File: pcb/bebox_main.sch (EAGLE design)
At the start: 29 parts, among them J1 SJ-435107RS, J2 SJ-435107RS, J4 SJ-435107RS, J6 PJ-102AH, P1 OSTTE020104, P2 OSTTE020104, P3 OSTTE020104, P4 OSTTE020104, P5 OSTTE020104, T1 TIP122, T2 TIP122, T3 TIP122, T4 TIP122, T5 TIP122

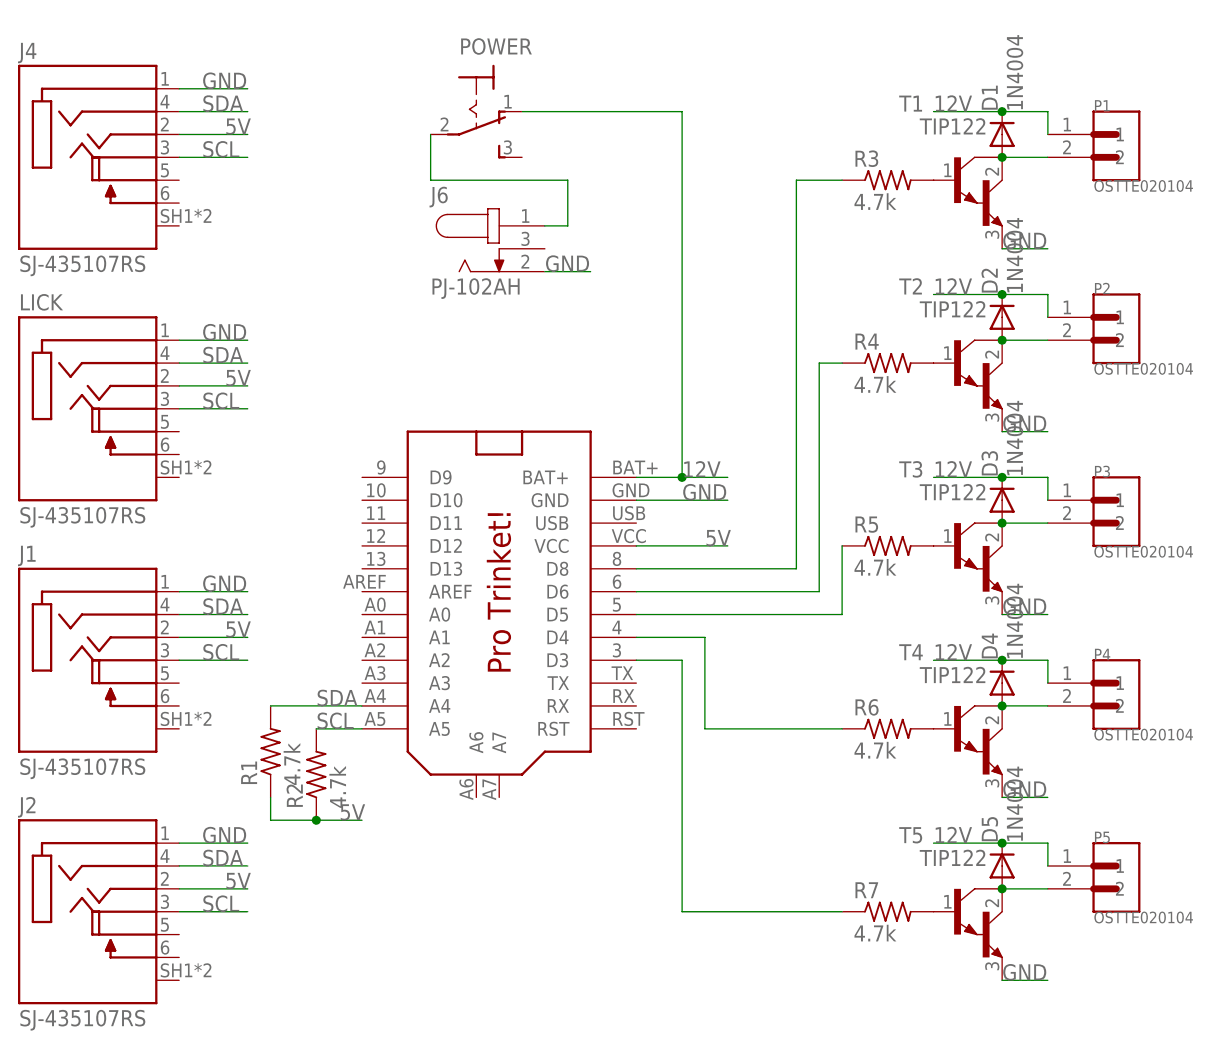
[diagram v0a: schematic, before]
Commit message: Updated the boards.
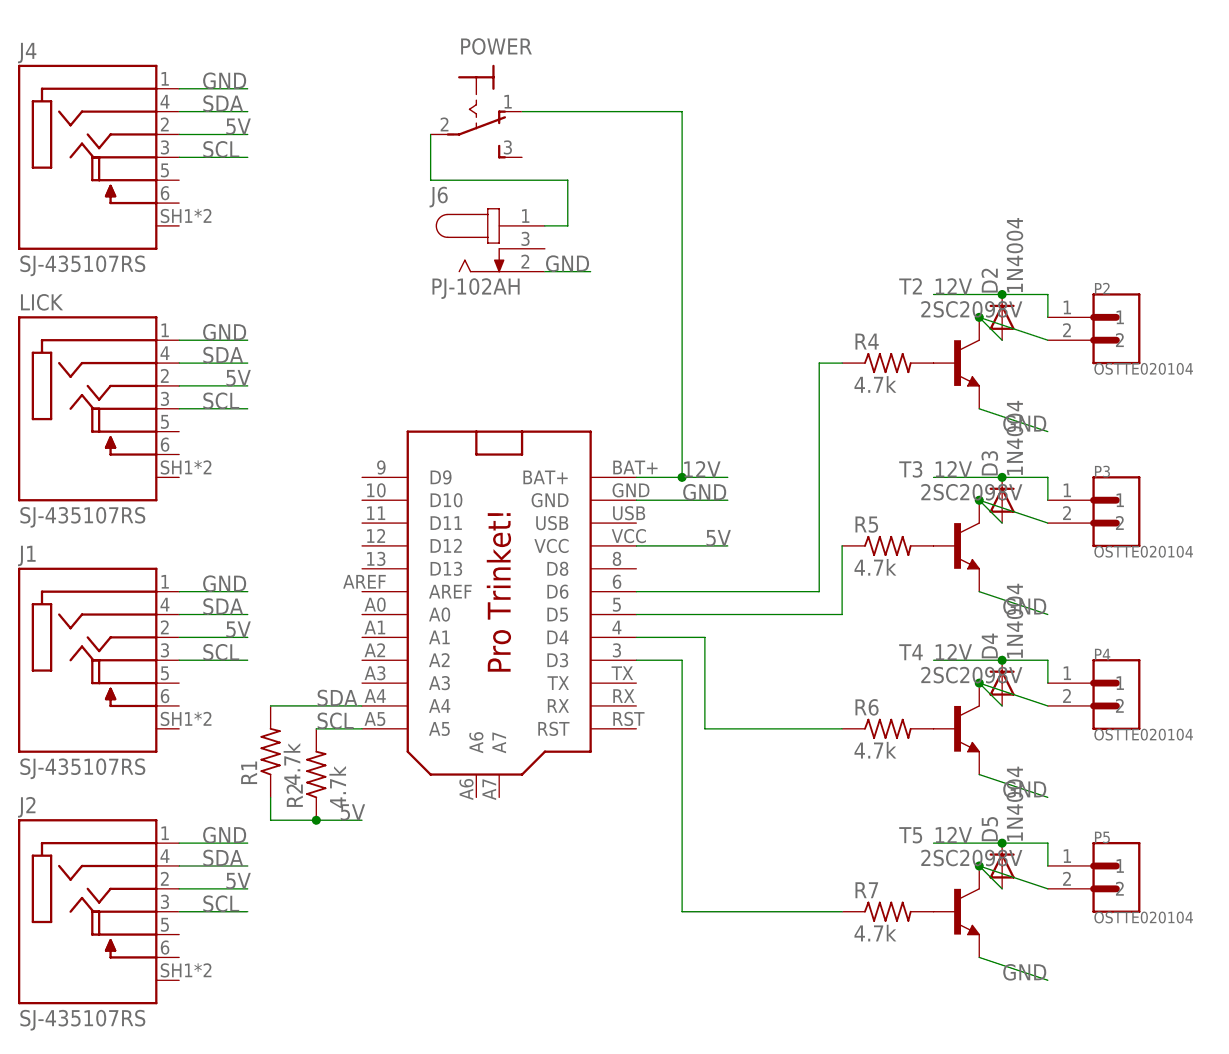
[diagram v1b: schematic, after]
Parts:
- removed D1: 1N4004, adafruit:1N4004
- removed P1: OSTTE020104, OSTTE020104:OSTTE020104
- removed R3: 4.7k, rcl:R-US_0207/10
- removed T1: TIP122, transistor-neu-to92:TIP122
- T2, T3, T4, T5: value TIP122 -> 2SC2098V; device transistor-neu-to92:TIP122 -> transistor:2SC2098V
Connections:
- removed net N$16: R3.1, U$1.D8
- removed net N$2: R3.2, T1.B
- removed net N$3: D1.A, P1.2, T1.C
- net 12V: no longer D1.C, P1.1
- net GND: no longer T1.E
